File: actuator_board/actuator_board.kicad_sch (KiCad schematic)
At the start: 33 parts, among them J1 Conn_01x10_Socket, J2 Conn_01x02_Socket, U1 113991054, U2 MCP4018T-103E/LTY, U3 TCA9548APWR, U4 MCP4018T-103E/LTY, U5 MCP4018T-103E/LTY, U6 MCP4018T-103E/LTY, U7 MCP4018T-103E/LTY, U8 STLQ015M33R

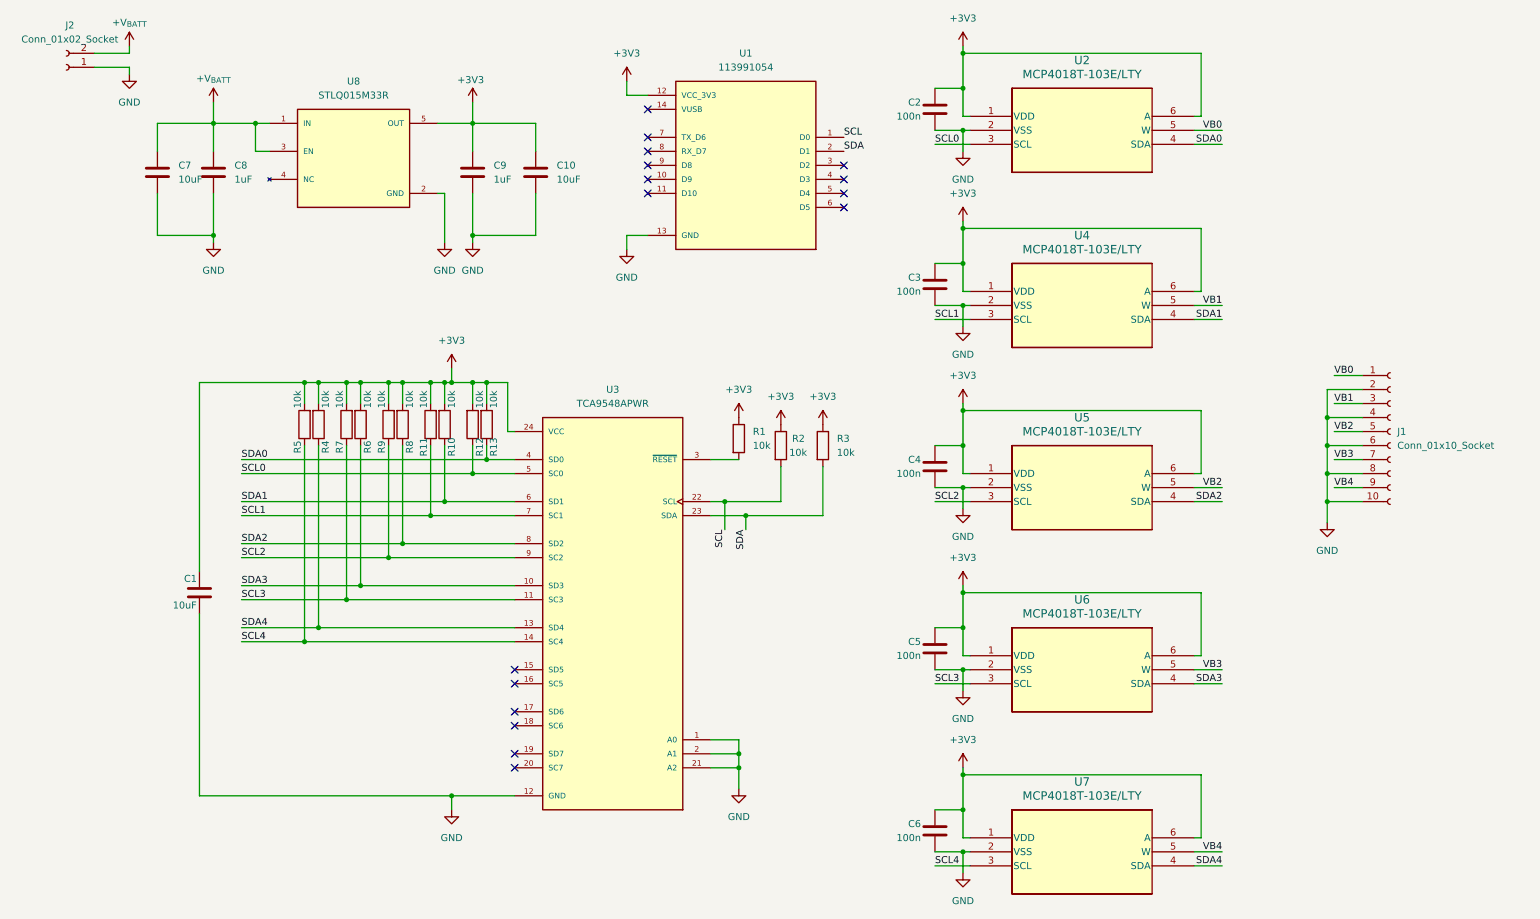
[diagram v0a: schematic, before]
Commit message: Finished actuator board.
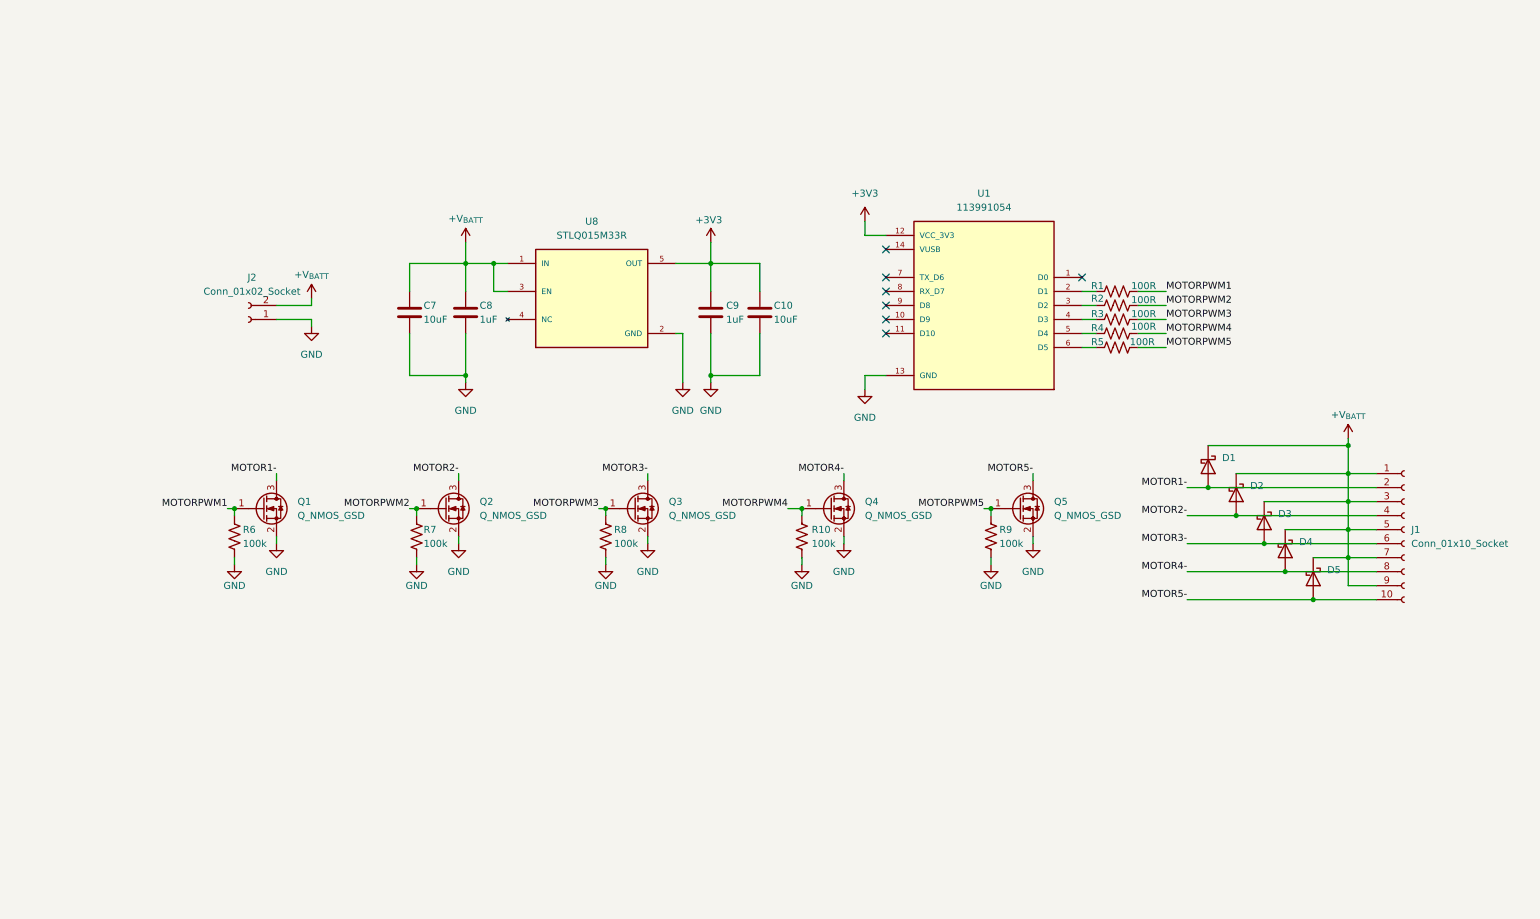
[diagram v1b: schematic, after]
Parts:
- removed C1: 10uF, Capacitor_SMD:C_0805_2012Metric, symbol Device:C
- removed C2, C3, C4, C5, C6: 100n, Capacitor_SMD:C_0805_2012Metric, symbol Device:C
- removed R1, R10, R11, R12, R13, R2, R3, R4, R5, R6, R7, R8, R9: 10k, Resistor_SMD:R_0805_2012Metric, symbol Device:R
- removed U2, U4, U5, U6, U7: MCP4018T-103E/LTY, mcp4018:SC70-6_LT_MCH, symbol 2025-10-21_01-01-03:MCP4018T-103E_LTY
- removed U3: TCA9548APWR, TCA9548APWR:SOP65P640X120-24N, symbol TCA9548APWR:TCA9548APWR
- added D1, D2, D3, D4, D5: D_Schottky, PMEG2010EH_115:DIO_PMEG3020EH_115, symbol Device:D_Schottky
- added Q1, Q2, Q3, Q4, Q5: Q_NMOS_GSD, IRLML6344TRPBF:TRANS_IRLML6344TRPBF, symbol Transistor_FET:Q_NMOS_GSD
- added R1, R2, R3, R4, R5: 100R, Resistor_SMD:R_0805_2012Metric_Pad1.20x1.40mm_HandSolder, symbol Device:R_US
- added R10, R6, R7, R8, R9: 100k, Resistor_SMD:R_0805_2012Metric_Pad1.20x1.40mm_HandSolder, symbol Device:R_US
- C10, C7, C8, C9: footprint Capacitor_SMD:C_0805_2012Metric -> Capacitor_SMD:C_0805_2012Metric_Pad1.18x1.45mm_HandSolder
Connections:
- net VB0 is gone; now on net +V_{BATT}: J1.1 (Pin_1)
- net VB1 is gone; now on net +V_{BATT}: J1.3 (Pin_3)
- net VB2 is gone; now on net +V_{BATT}: J1.5 (Pin_5)
- net VB3 is gone; now on net +V_{BATT}: J1.7 (Pin_7)
- net VB4 is gone; now on net +V_{BATT}: J1.9 (Pin_9)
- net +V_{BATT}: now also D1.1 (K), D2.1 (K), D3.1 (K), D4.1 (K), D5.1 (K)
- net GND: now also Q1.2 (S), Q2.2 (S), Q3.2 (S), Q4.2 (S), Q5.2 (S), R10.2, R6.2, R7.2, R8.2, R9.2; no longer J1.10 (Pin_10), J1.2 (Pin_2), J1.4 (Pin_4), J1.6 (Pin_6), J1.8 (Pin_8)
- net at U1.3 (D2): now also R2.1
- net at U1.4 (D3): now also R3.1
- net at U1.5 (D4): now also R4.1
- net at U1.6 (D5): now also R5.1
- net SCL: no longer names the net of U1.1 (D0)
- net SDA: no longer names the net of U1.2 (D1)
- net SDA: now also R1.1
- new net MOTOR1-: D1.2 (A), J1.2 (Pin_2), Q1.3 (D)
- new net MOTOR2-: D2.2 (A), J1.4 (Pin_4), Q2.3 (D)
- new net MOTOR3-: D3.2 (A), J1.6 (Pin_6), Q3.3 (D)
- new net MOTOR4-: D4.2 (A), J1.8 (Pin_8), Q4.3 (D)
- new net MOTOR5-: D5.2 (A), J1.10 (Pin_10), Q5.3 (D)
- new net MOTORPWM1: Q1.1 (G), R1.2, R6.1
- new net MOTORPWM2: Q2.1 (G), R2.2, R7.1
- new net MOTORPWM3: Q3.1 (G), R3.2, R8.1
- new net MOTORPWM4: Q4.1 (G), R10.1, R4.2
- new net MOTORPWM5: Q5.1 (G), R5.2, R9.1
- no-connect marks 16 -> 7
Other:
- moved on the sheet: C10, C7, C8, C9, J1, J2, U1, U8
